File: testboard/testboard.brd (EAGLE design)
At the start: 9.8 x 11.4 mm, 1 part

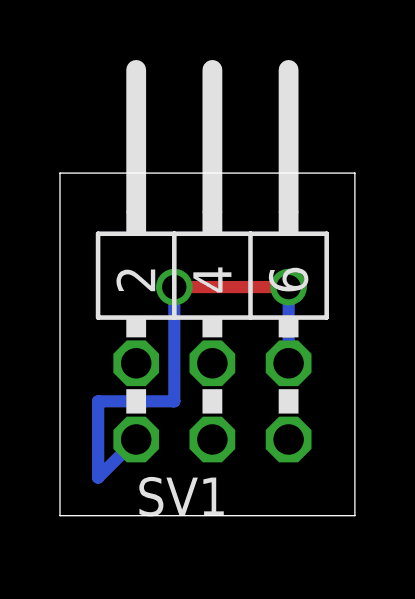
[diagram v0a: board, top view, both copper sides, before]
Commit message: Updating test board
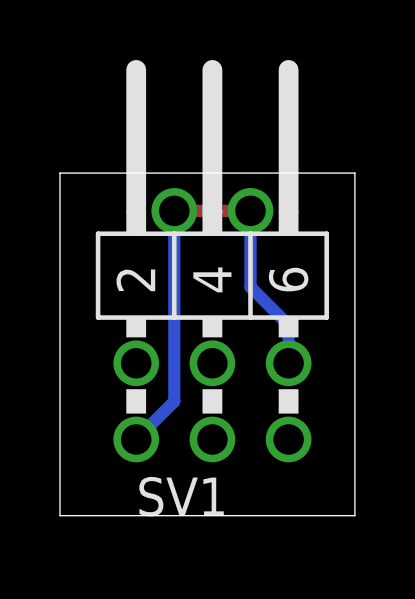
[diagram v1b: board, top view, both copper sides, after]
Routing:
- net N$1: track 17.0 -> 16.3 mm
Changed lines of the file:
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@@
 <contactref element="SV1" pad="1"/>
 <contactref element="SV1" pad="6"/>
-<wire x1="2.54" y1="2.54" x2="1.27" y2="1.27" width="0.4064" layer="16"/>
-<wire x1="1.27" y1="1.27" x2="1.27" y2="3.81" width="0.4064" layer="16"/>
-<wire x1="1.27" y1="3.81" x2="3.81" y2="3.81" width="0.4064" layer="16"/>
-<wire x1="3.81" y1="3.81" x2="3.81" y2="7.62" width="0.4064" layer="16"/>
-<via x="3.81" y="7.62" extent="1-16" drill="0.8128"/>
-<wire x1="3.81" y1="7.62" x2="7.62" y2="7.62" width="0.4064" layer="1"/>
-<via x="7.62" y="7.62" extent="1-16" drill="0.8128"/>
-<wire x1="7.62" y1="7.62" x2="7.62" y2="5.08" width="0.4064" layer="16"/>
+<wire x1="7.62" y1="5.08" x2="7.62" y2="6.35" width="0.4064" layer="16"/>
+<wire x1="7.62" y1="6.35" x2="6.35" y2="7.62" width="0.4064" layer="16"/>
+<wire x1="6.35" y1="7.62" x2="6.35" y2="10.16" width="0.4064" layer="16"/>
+<via x="6.35" y="10.16" extent="1-16" drill="1.016"/>
+<wire x1="6.35" y1="10.16" x2="3.81" y2="10.16" width="0.4064" layer="1"/>
+<via x="3.81" y="10.16" extent="1-16" drill="1.016"/>
+<wire x1="3.81" y1="10.16" x2="3.81" y2="3.81" width="0.4064" layer="16"/>
+<wire x1="3.81" y1="3.81" x2="2.54" y2="2.54" width="0.4064" layer="16"/>
 </signal>
 </signals>
